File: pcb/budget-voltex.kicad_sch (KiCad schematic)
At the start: 10 parts

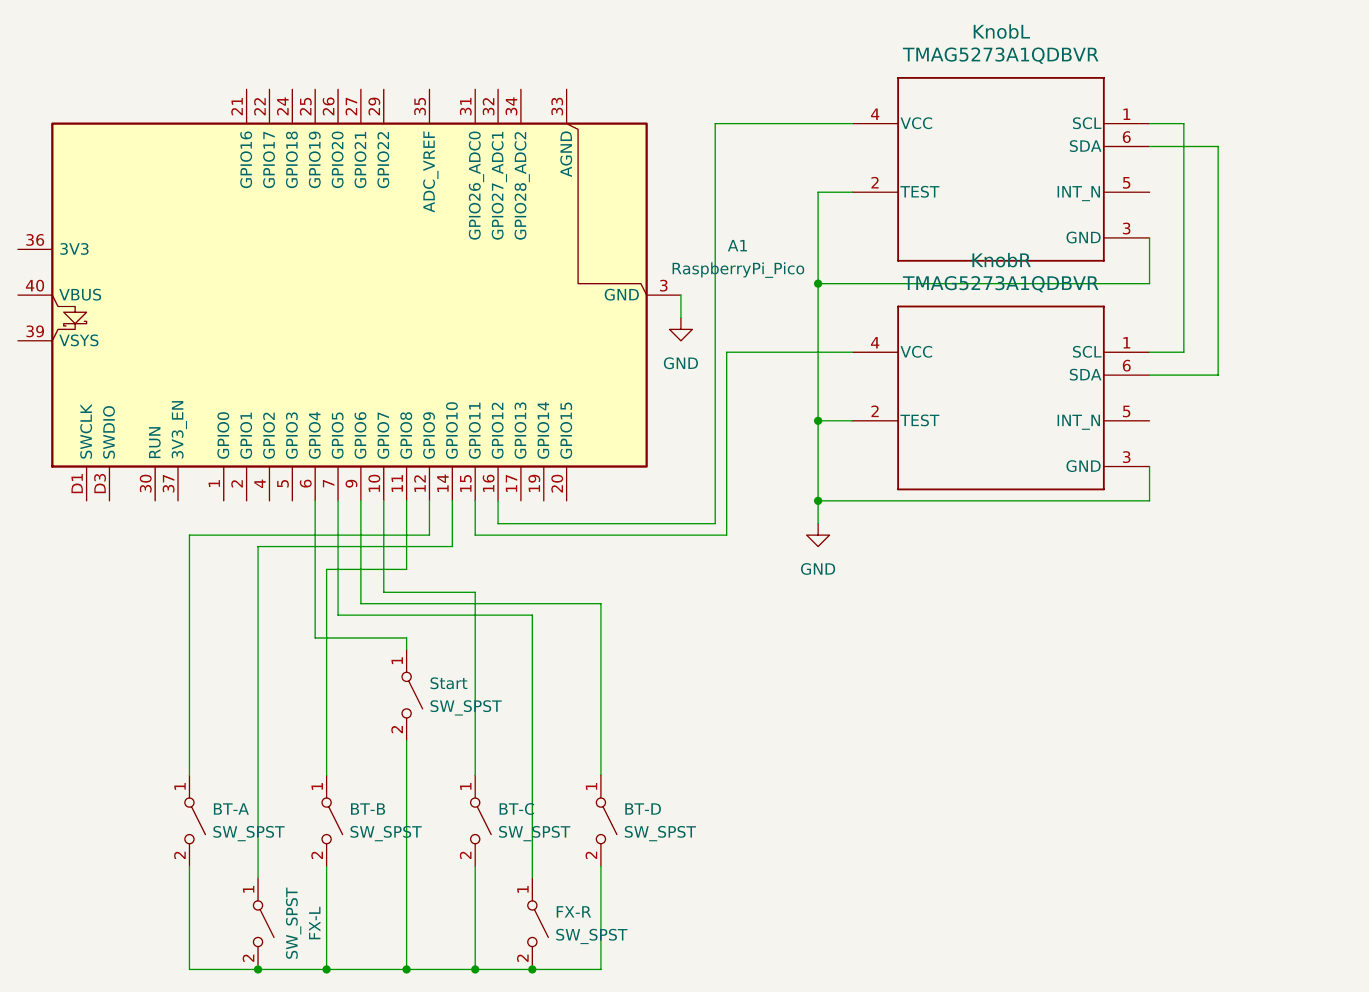
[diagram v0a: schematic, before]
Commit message: put elements on pcb
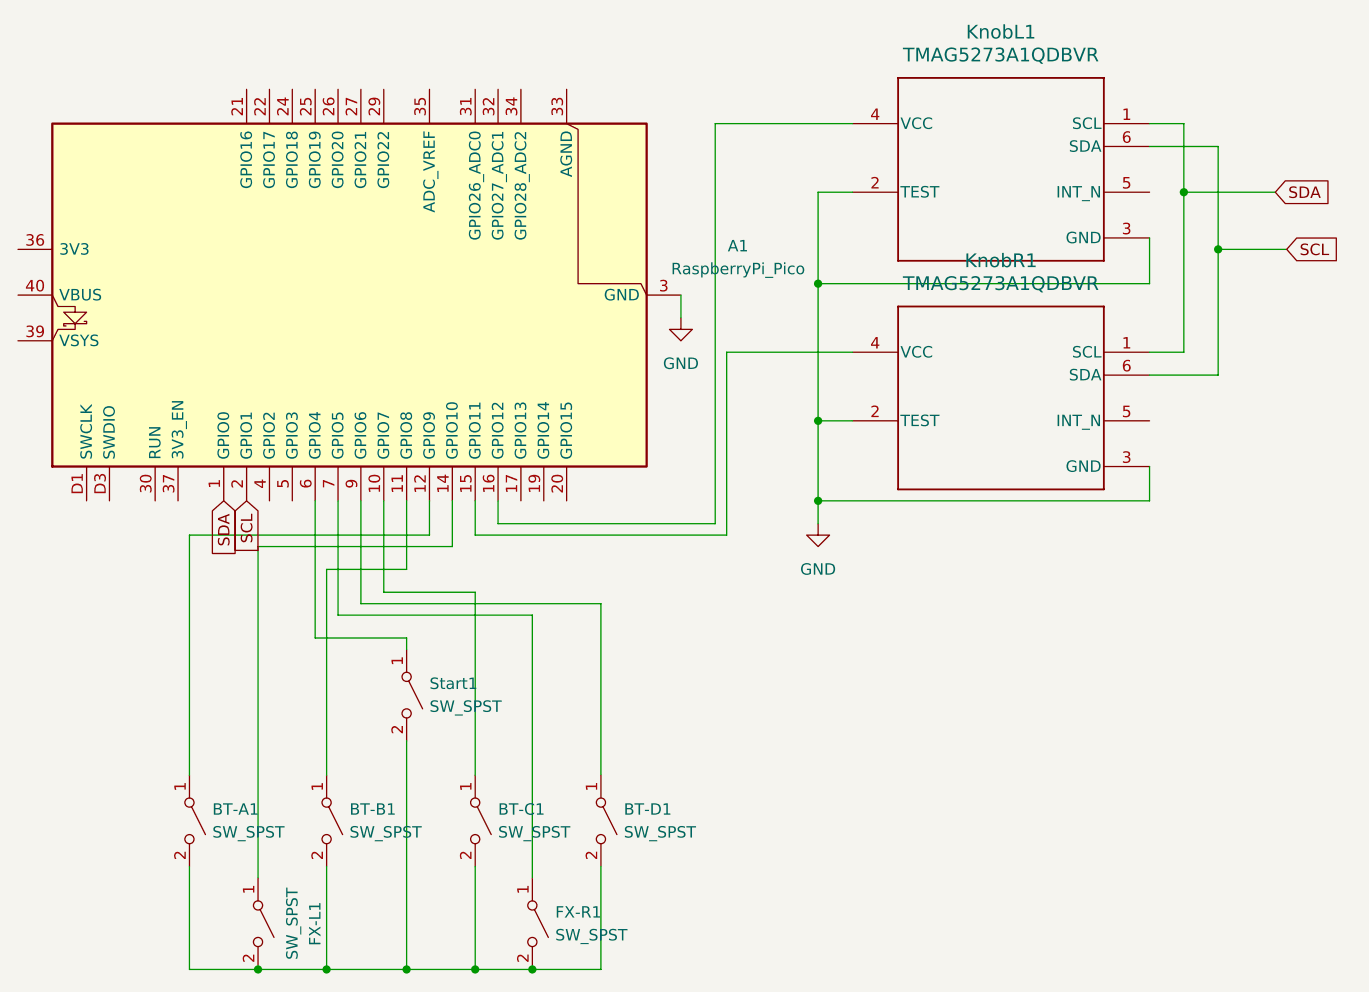
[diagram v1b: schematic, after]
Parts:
- BT-A1: renamed from BT-A; footprint (none) -> Button_Switch_Keyboard:SW_Cherry_MX_1.00u_PCB
- BT-B1: renamed from BT-B; footprint (none) -> Button_Switch_Keyboard:SW_Cherry_MX_1.00u_PCB
- BT-C1: renamed from BT-C; footprint (none) -> Button_Switch_Keyboard:SW_Cherry_MX_1.00u_PCB
- BT-D1: renamed from BT-D; footprint (none) -> Button_Switch_Keyboard:SW_Cherry_MX_1.00u_PCB
- FX-L1: renamed from FX-L; footprint (none) -> Button_Switch_Keyboard:SW_Cherry_MX_1.00u_PCB
- FX-R1: renamed from FX-R; footprint (none) -> Button_Switch_Keyboard:SW_Cherry_MX_1.00u_PCB
- Start1: renamed from Start; footprint (none) -> Button_Switch_Keyboard:SW_Cherry_MX_1.00u_PCB
- renumbered KnobL to KnobL1, KnobR to KnobR1
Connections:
- net SDA: now reaches KnobL1.1 (SCL), KnobR1.1 (SCL)
- net SDA: now also A1.1 (GPIO0)
- net SCL: now reaches KnobL1.6 (SDA), KnobR1.6 (SDA)
- net SCL: now also A1.2 (GPIO1)
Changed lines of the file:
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@@
 	(paper "A4")
+	(junction
+		(at 182.88 77.47)
+		(diameter 0)
+		(color 0 0 0 0)
+	)
 	(junction
 		(at 76.2 157.48)
@@
 	)
 	(junction
+		(at 179.07 71.12)
+		(diameter 0)
+		(color 0 0 0 0)
+	)
+	(junction
 		(at 106.68 157.48)
 		(diameter 0)
@@
 	(wire
 		(pts
+			(xy 179.07 71.12) (xy 189.23 71.12)
+		)
+		(stroke
+			(width 0)
+			(type default)
+		)
+	)
+	(wire
+		(pts
 			(xy 92.71 113.03) (xy 92.71 105.41)
 		)
@@
 	(wire
 		(pts
+			(xy 179.07 71.12) (xy 179.07 63.5)
+		)
+		(stroke
+			(width 0)
+			(type default)
+		)
+	)
+	(wire
+		(pts
 			(xy 83.82 157.48) (xy 83.82 146.05)
 		)
@@
 	(wire
 		(pts
+			(xy 182.88 77.47) (xy 182.88 66.04)
+		)
+		(stroke
+			(width 0)
+			(type default)
+		)
+	)
+	(wire
+		(pts
 			(xy 82.55 105.41) (xy 82.55 120.65)
 		)
@@
 	(wire
 		(pts
-			(xy 182.88 91.44) (xy 182.88 66.04)
+			(xy 182.88 91.44) (xy 182.88 77.47)
 		)
 		(stroke
@@
 	(wire
 		(pts
-			(xy 179.07 88.9) (xy 179.07 63.5)
+			(xy 179.07 88.9) (xy 179.07 71.12)
 		)
 		(stroke
@@
 	(wire
 		(pts
+			(xy 182.88 77.47) (xy 190.5 77.47)
+		)
+		(stroke
+			(width 0)
+			(type default)
+		)
+	)
+	(wire
+		(pts
 			(xy 100.33 115.57) (xy 90.17 115.57)
 		)
@@
 			(width 0)
 			(type default)
+		)
+	)
+	(global_label "SCL"
+		(shape input)
+		(at 74.93 105.41 270)
+		(fields_autoplaced yes)
+		(effects
+			(font
+				(size 1.27 1.27)
+			)
+			(justify right)
+		)
+		(property "Intersheetrefs" "${INTERSHEET_REFS}"
+			(at 74.93 111.9028 90)
+			(effects
+				(font
+					(size 1.27 1.27)
+				)
+				(justify right)
+				(hide yes)
+			)
+		)
+	)
+	(global_label "SCL"
+		(shape input)
+		(at 190.5 77.47 0)
+		(fields_autoplaced yes)
+		(effects
+			(font
+				(size 1.27 1.27)
+			)
+			(justify left)
+		)
+		(property "Intersheetrefs" "${INTERSHEET_REFS}"
+			(at 196.9928 77.47 0)
+			(effects
+				(font
+					(size 1.27 1.27)
+				)
+				(justify left)
+				(hide yes)
+			)
+		)
+	)
+	(global_label "SDA"
+		(shape input)
+		(at 72.39 105.41 270)
+		(fields_autoplaced yes)
+		(effects
+			(font
+				(size 1.27 1.27)
+			)
+			(justify right)
+		)
+		(property "Intersheetrefs" "${INTERSHEET_REFS}"
+			(at 72.39 111.9633 90)
+			(effects
+				(font
+					(size 1.27 1.27)
+				)
+				(justify right)
+				(hide yes)
+			)
+		)
+	)
+	(global_label "SDA"
+		(shape input)
+		(at 189.23 71.12 0)
+		(fields_autoplaced yes)
+		(effects
+			(font
+				(size 1.27 1.27)
+			)
+			(justify left)
+		)
+		(property "Intersheetrefs" "${INTERSHEET_REFS}"
+			(at 195.7833 71.12 0)
+			(effects
+				(font
+					(size 1.27 1.27)
+				)
+				(justify left)
+				(hide yes)
+			)
 		)
 	)
@@
 		(dnp no)
 		(fields_autoplaced yes)
-		(property "Reference" "KnobL"
+		(property "Reference" "KnobL1"
 			(at 158.75 53.34 0)
 			(effects
@@
 			(project "sdvx-slim"
 				(path "/f61fff6d-f3d6-4025-b479-f6b910efe925"
-					(reference "KnobL")
+					(reference "KnobL1")
 					(unit 1)
 				)
@@
 		(on_board yes)
 		(dnp no)
-		(property "Reference" "FX-L"
+		(property "Reference" "FX-L1"
 			(at 82.55 152.4 0)
 			(effects
@@
 			)
 		)
-		(property "Footprint" ""
+		(property "Footprint" "Button_Switch_Keyboard:SW_Cherry_MX_1.00u_PCB"
 			(at 76.2 152.4 0)
 			(effects
@@
 			(project "sdvx-slim"
 				(path "/f61fff6d-f3d6-4025-b479-f6b910efe925"
-					(reference "FX-L")
+					(reference "FX-L1")
 					(unit 1)
 				)
@@
 		(dnp no)
 		(fields_autoplaced yes)
-		(property "Reference" "Start"
+		(property "Reference" "Start1"
 			(at 95.25 125.7299 90)
 			(effects
@@
 			)
 		)
-		(property "Footprint" ""
+		(property "Footprint" "Button_Switch_Keyboard:SW_Cherry_MX_1.00u_PCB"
 			(at 92.71 127 0)
 			(effects
@@
 			(project "sdvx-slim"
 				(path "/f61fff6d-f3d6-4025-b479-f6b910efe925"
-					(reference "Start")
+					(reference "Start1")
 					(unit 1)
 				)
@@
 		(dnp no)
 		(fields_autoplaced yes)
-		(property "Reference" "BT-D"
+		(property "Reference" "BT-D1"
 			(at 116.84 139.6999 90)
 			(effects
@@
 			)
 		)
-		(property "Footprint" ""
+		(property "Footprint" "Button_Switch_Keyboard:SW_Cherry_MX_1.00u_PCB"
 			(at 114.3 140.97 0)
 			(effects
@@
 			(project "sdvx-slim"
 				(path "/f61fff6d-f3d6-4025-b479-f6b910efe925"
-					(reference "BT-D")
+					(reference "BT-D1")
 					(unit 1)
 				)
@@
 		(dnp no)
 		(fields_autoplaced yes)
-		(property "Reference" "KnobR"
+		(property "Reference" "KnobR1"
 			(at 158.75 78.74 0)
 			(effects
@@
 			(project ""
 				(path "/f61fff6d-f3d6-4025-b479-f6b910efe925"
-					(reference "KnobR")
+					(reference "KnobR1")
 					(unit 1)
 				)
@@
 		(dnp no)
 		(fields_autoplaced yes)
-		(property "Reference" "BT-A"
+		(property "Reference" "BT-A1"
 			(at 71.12 139.6999 90)
 			(effects
@@
 			)
 		)
-		(property "Footprint" ""
+		(property "Footprint" "Button_Switch_Keyboard:SW_Cherry_MX_1.00u_PCB"
 			(at 68.58 140.97 0)
 			(effects
@@
 			(project ""
 				(path "/f61fff6d-f3d6-4025-b479-f6b910efe925"
-					(reference "BT-A")
+					(reference "BT-A1")
 					(unit 1)
 				)
@@
 		(dnp no)
 		(fields_autoplaced yes)
-		(property "Reference" "BT-C"
+		(property "Reference" "BT-C1"
 			(at 102.87 139.6999 90)
 			(effects
@@
 			)
 		)
-		(property "Footprint" ""
+		(property "Footprint" "Button_Switch_Keyboard:SW_Cherry_MX_1.00u_PCB"
 			(at 100.33 140.97 0)
 			(effects
@@
 			(project "sdvx-slim"
 				(path "/f61fff6d-f3d6-4025-b479-f6b910efe925"
-					(reference "BT-C")
+					(reference "BT-C1")
 					(unit 1)
 				)
@@
 		(dnp no)
 		(fields_autoplaced yes)
-		(property "Reference" "BT-B"
+		(property "Reference" "BT-B1"
 			(at 86.36 139.6999 90)
 			(effects
@@
 			)
 		)
-		(property "Footprint" ""
+		(property "Footprint" "Button_Switch_Keyboard:SW_Cherry_MX_1.00u_PCB"
 			(at 83.82 140.97 0)
 			(effects
@@
 			(project "sdvx-slim"
 				(path "/f61fff6d-f3d6-4025-b479-f6b910efe925"
-					(reference "BT-B")
+					(reference "BT-B1")
 					(unit 1)
 				)
@@
 		(dnp no)
 		(fields_autoplaced yes)
-		(property "Reference" "FX-R"
+		(property "Reference" "FX-R1"
 			(at 109.22 151.1299 90)
 			(effects
@@
 			)
 		)
-		(property "Footprint" ""
+		(property "Footprint" "Button_Switch_Keyboard:SW_Cherry_MX_1.00u_PCB"
 			(at 106.68 152.4 0)
 			(effects
@@
 			(project "sdvx-slim"
 				(path "/f61fff6d-f3d6-4025-b479-f6b910efe925"
-					(reference "FX-R")
+					(reference "FX-R1")
 					(unit 1)
 				)
